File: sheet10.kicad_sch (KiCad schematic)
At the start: 69 parts, among them J1 ISA Bus connector, J10 AT POWER CONNECTOR, J2 ISA Bus connector, J3 ISA Bus connector, J4 ISA Bus connector, J5 ISA Bus connector, J6 ISA Bus connector, J7 ISA Bus connector, J8 ISA Bus connector

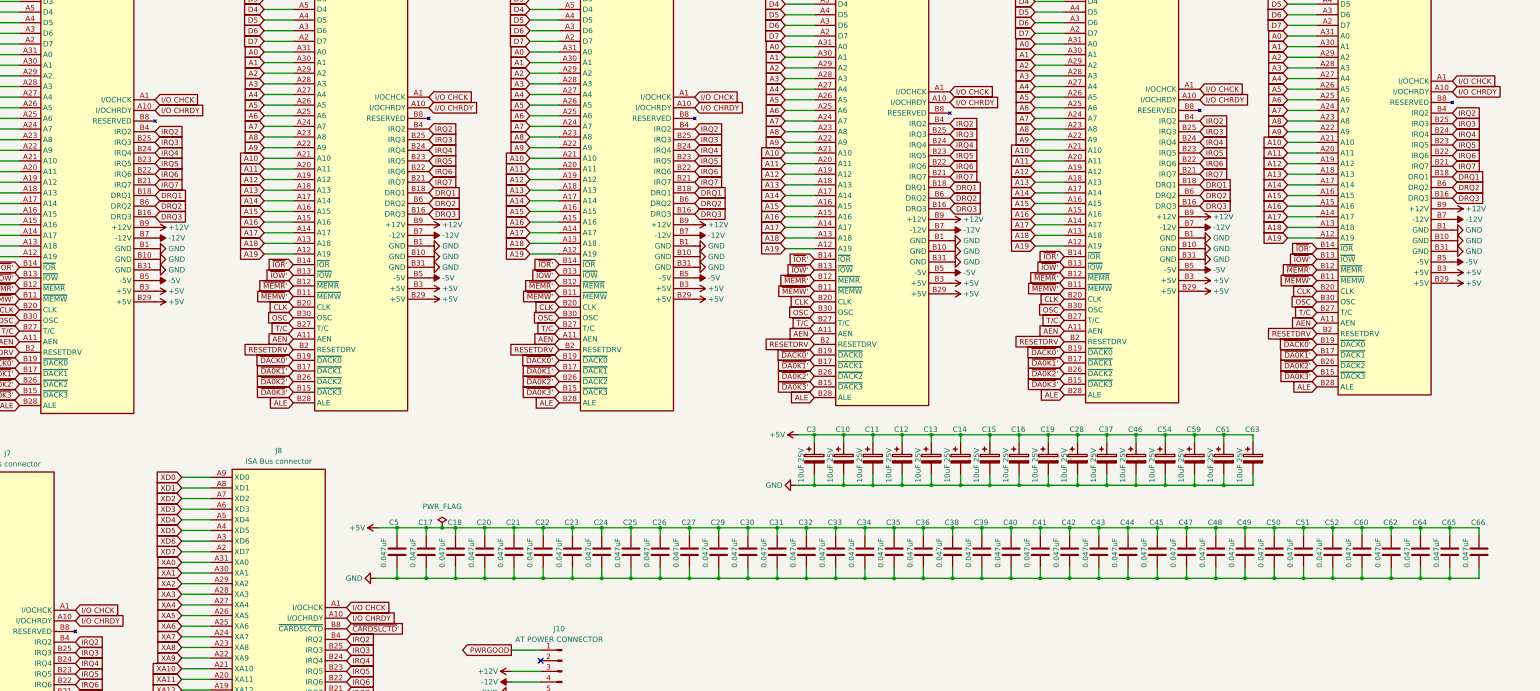
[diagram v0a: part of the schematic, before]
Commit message: Version 1.0 fix
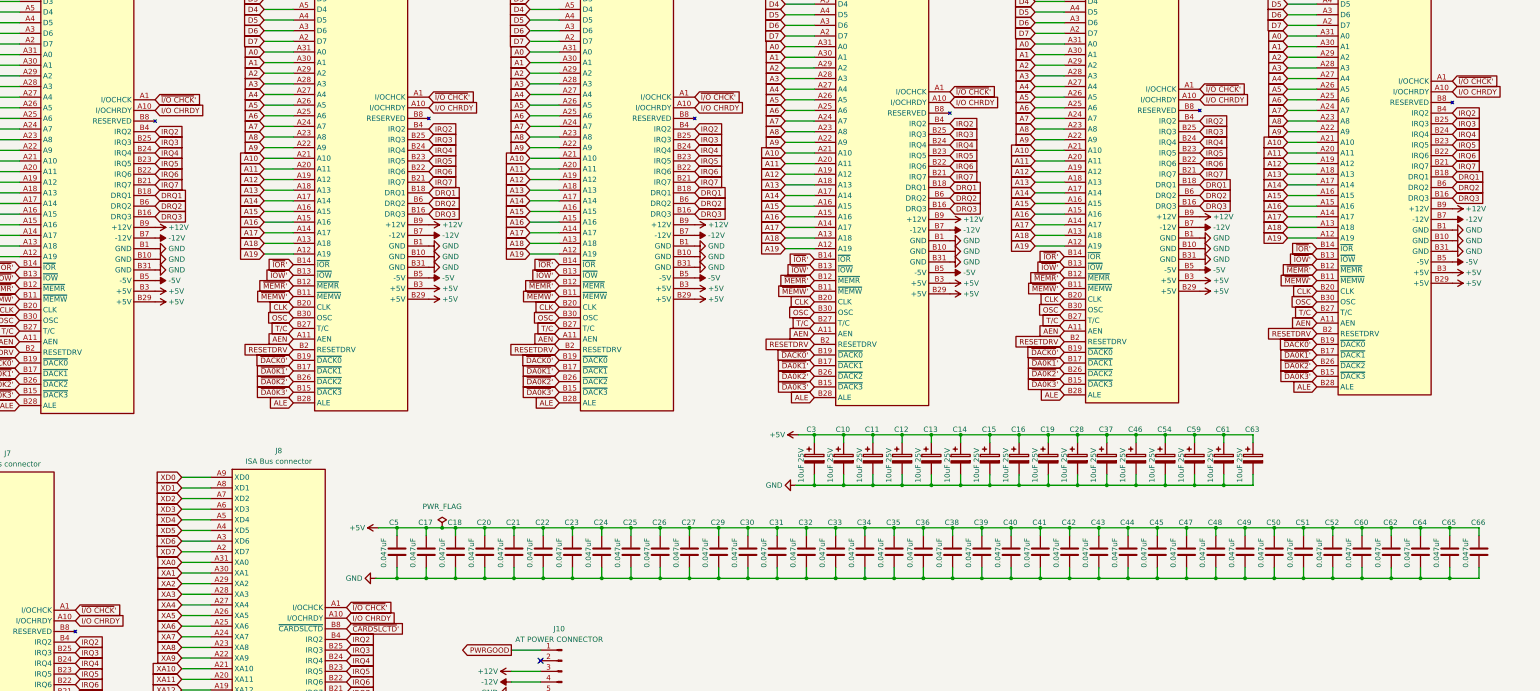
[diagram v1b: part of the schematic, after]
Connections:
- net I/O CHCK renamed ~{I/O CHCK}'
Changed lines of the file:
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@@
     )
   )
-  (global_label "I{slash}O CHCK" (shape input) (at 394.335 59.69 0) (fields_autoplaced)
-    (effects (font (size 1.27 1.27)) (justify left))
-    (property "Intersheetrefs" "${INTERSHEET_REFS}" (at 406.6941 59.69 0)
+  (global_label "~{I{slash}O CHCK}'" (shape input) (at 394.335 59.69 0) (fields_autoplaced)
+    (effects (font (size 1.27 1.27)) (justify left))
+    (property "Intersheetrefs" "${INTERSHEET_REFS}" (at 407.2989 59.69 0)
       (effects (font (size 1.27 1.27)) (justify left) hide)
     )
@@
     )
   )
-  (global_label "I{slash}O CHCK" (shape input) (at 65.405 186.055 0) (fields_autoplaced)
-    (effects (font (size 1.27 1.27)) (justify left))
-    (property "Intersheetrefs" "${INTERSHEET_REFS}" (at 77.7641 186.055 0)
+  (global_label "~{I{slash}O CHCK}'" (shape input) (at 65.405 186.055 0) (fields_autoplaced)
+    (effects (font (size 1.27 1.27)) (justify left))
+    (property "Intersheetrefs" "${INTERSHEET_REFS}" (at 78.3689 186.055 0)
       (effects (font (size 1.27 1.27)) (justify left) hide)
     )
@@
     )
   )
-  (global_label "I{slash}O CHCK" (shape input) (at 149.86 63.5 0) (fields_autoplaced)
-    (effects (font (size 1.27 1.27)) (justify left))
-    (property "Intersheetrefs" "${INTERSHEET_REFS}" (at 162.2191 63.5 0)
+  (global_label "~{I{slash}O CHCK}'" (shape input) (at 149.86 63.5 0) (fields_autoplaced)
+    (effects (font (size 1.27 1.27)) (justify left))
+    (property "Intersheetrefs" "${INTERSHEET_REFS}" (at 162.8239 63.5 0)
       (effects (font (size 1.27 1.27)) (justify left) hide)
     )
@@
     )
   )
-  (global_label "I{slash}O CHCK" (shape input) (at 84.455 64.135 0) (fields_autoplaced)
-    (effects (font (size 1.27 1.27)) (justify left))
-    (property "Intersheetrefs" "${INTERSHEET_REFS}" (at 96.8141 64.135 0)
+  (global_label "~{I{slash}O CHCK}'" (shape input) (at 84.455 64.135 0) (fields_autoplaced)
+    (effects (font (size 1.27 1.27)) (justify left))
+    (property "Intersheetrefs" "${INTERSHEET_REFS}" (at 97.4189 64.135 0)
       (effects (font (size 1.27 1.27)) (justify left) hide)
     )
@@
     )
   )
-  (global_label "I{slash}O CHCK" (shape input) (at 130.175 185.42 0) (fields_autoplaced)
-    (effects (font (size 1.27 1.27)) (justify left))
-    (property "Intersheetrefs" "${INTERSHEET_REFS}" (at 142.5341 185.42 0)
+  (global_label "~{I{slash}O CHCK}'" (shape input) (at 130.175 185.42 0) (fields_autoplaced)
+    (effects (font (size 1.27 1.27)) (justify left))
+    (property "Intersheetrefs" "${INTERSHEET_REFS}" (at 143.1389 185.42 0)
       (effects (font (size 1.27 1.27)) (justify left) hide)
     )
@@
     )
   )
-  (global_label "I{slash}O CHCK" (shape input) (at 213.36 63.5 0) (fields_autoplaced)
-    (effects (font (size 1.27 1.27)) (justify left))
-    (property "Intersheetrefs" "${INTERSHEET_REFS}" (at 225.7191 63.5 0)
+  (global_label "~{I{slash}O CHCK}'" (shape input) (at 213.36 63.5 0) (fields_autoplaced)
+    (effects (font (size 1.27 1.27)) (justify left))
+    (property "Intersheetrefs" "${INTERSHEET_REFS}" (at 226.3239 63.5 0)
       (effects (font (size 1.27 1.27)) (justify left) hide)
     )
@@
     )
   )
-  (global_label "I{slash}O CHCK" (shape input) (at 274.32 62.23 0) (fields_autoplaced)
-    (effects (font (size 1.27 1.27)) (justify left))
-    (property "Intersheetrefs" "${INTERSHEET_REFS}" (at 286.6791 62.23 0)
+  (global_label "~{I{slash}O CHCK}'" (shape input) (at 274.32 62.23 0) (fields_autoplaced)
+    (effects (font (size 1.27 1.27)) (justify left))
+    (property "Intersheetrefs" "${INTERSHEET_REFS}" (at 287.2839 62.23 0)
       (effects (font (size 1.27 1.27)) (justify left) hide)
     )
@@
     )
   )
-  (global_label "I{slash}O CHCK" (shape input) (at 334.01 61.595 0) (fields_autoplaced)
-    (effects (font (size 1.27 1.27)) (justify left))
-    (property "Intersheetrefs" "${INTERSHEET_REFS}" (at 346.3691 61.595 0)
-      (effects (font (size 1.27 1.27)) (justify left) hide)
-    )
+  (global_label "~{I{slash}O CHCK}'" (shape input) (at 334.01 61.595 0) (fields_autoplaced)
+    (effects (font (size 1.27 1.27)) (justify left))
+    (property "Intersheetrefs" "${INTERSHEET_REFS}" (at 346.9739 61.595 0)
+      (effects (font (size 1.27 1.27)) (justify left) hide)
+    )
